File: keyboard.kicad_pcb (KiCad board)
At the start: 2 copper layers, 100 parts, among them J1 AudioJack4, J2 AudioJack4, SW1 , SW11 , SW12 , SW13 , SW14 , SW15 , SW16 , SW17 , SW18 RotaryEncoder_Switch, SW19 , SW2 , SW20 , SW21 , SW22 , SW23 , SW24 SW_PUSH, SW25 SW_PUSH, SW3 , SW4 , SW5 , SW6 , SW7 , SW8 , SW9 , U1 ProMicro

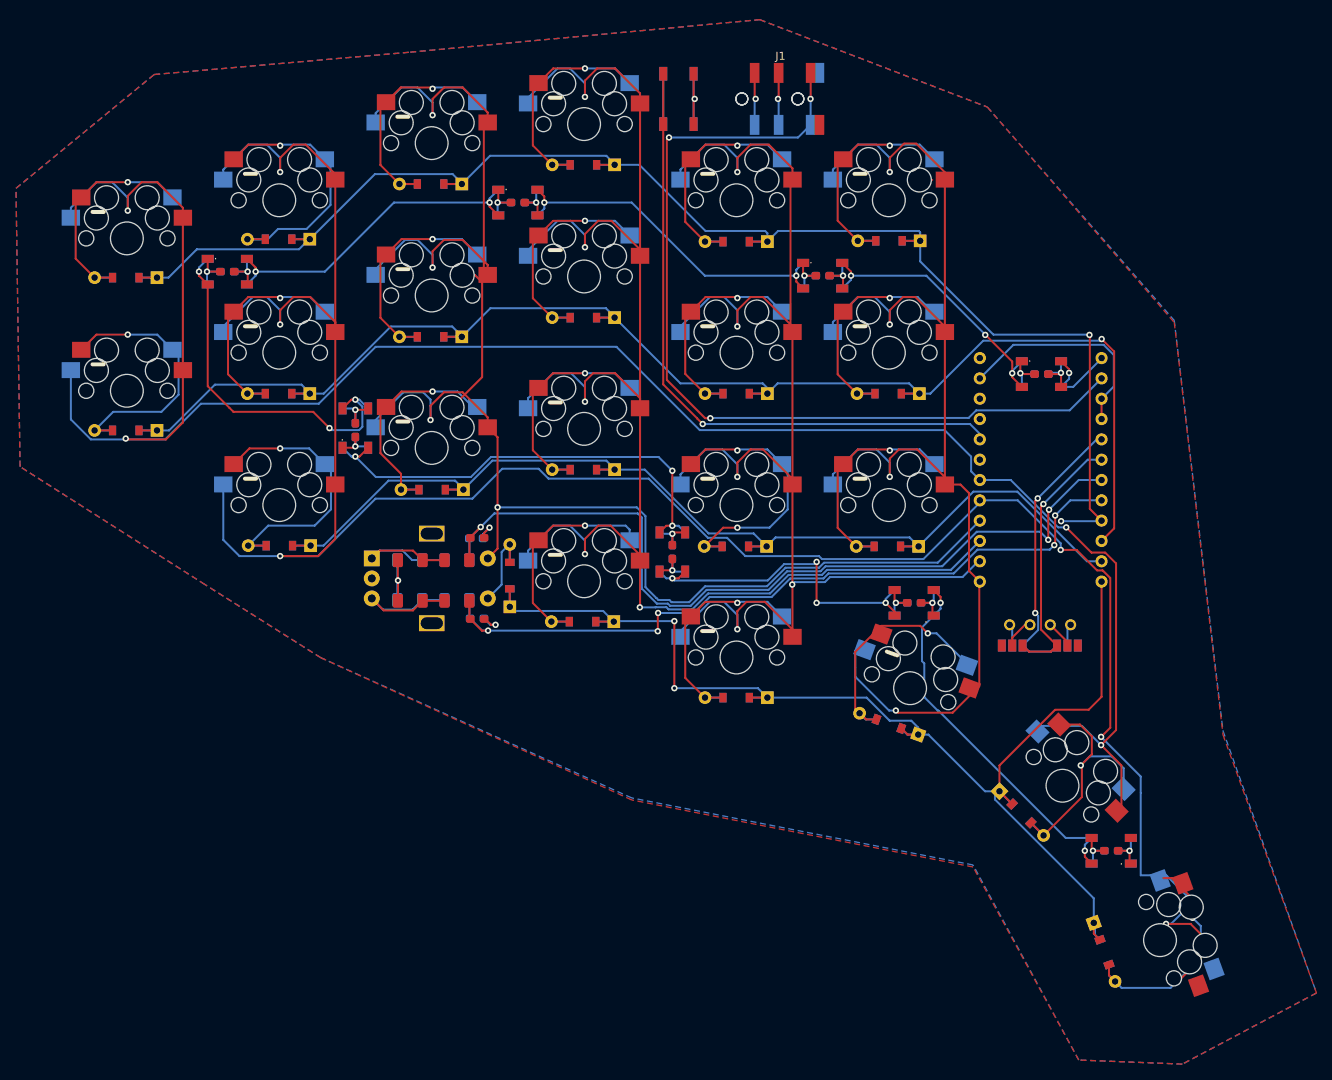
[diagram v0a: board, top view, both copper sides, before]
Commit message: wireless
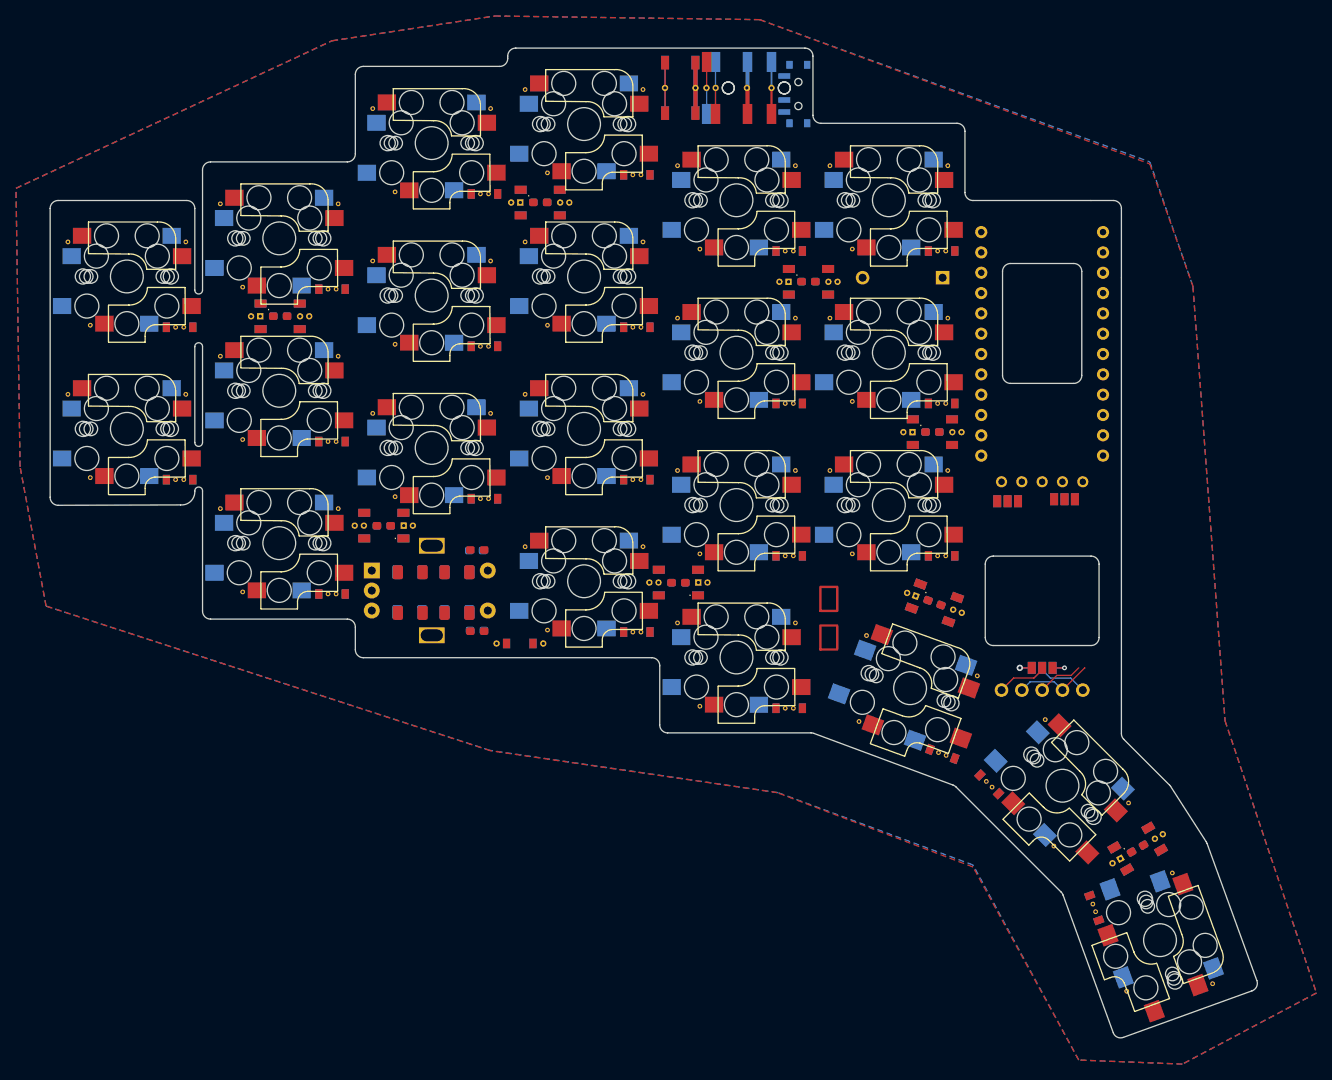
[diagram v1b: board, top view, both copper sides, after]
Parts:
- removed C10, C11, C12, C13, C14, C15, C16, C17, C18, C3, C4, C5, C6, C7, C8, C9: 0.1u, keyswitches:Cap_0603_Clean
- removed D10, D11, D12, D13, D14, D15, D16, D17, D18, D19, D20, D21, D22, D23: , keyswitches:REVERSIBLED_SOD-123
- removed D24, D25, D26, D27, D28, D29, D30, D31, D33, D34, D35, D36, D37, D38, D39, D40: , keyswitches:ledClean
- added J3: Conn_01x05, hb44:Pimoroni Haptic Buzz DRV2605L Driver, B.Cu at (152.1, 99.1)
- added JP5: SolderJumper_3_Open, keyswitches:jumperClean, B.Cu at (152.1, 106.7)
- added JP6: SolderJumper_3_Open, keyswitches:jumperClean, F.Cu at (152.1, 106.7)
- D1: footprint keyswitches:REVERSIBLED_SOD-123 -> hb44:SMD_SOD123
- D2, D3, D4, D5, D6, D7, D8, D9: value (none) -> WS2812B+Cap; footprint keyswitches:REVERSIBLED_SOD-123 -> hb44:SMD_WS2812B+Cap0603; moved to B.Cu
- J1: footprint keyswitches:jackClean -> hb44:SMD_3.5mm_TRRS; moved to B.Cu
- J2: value AudioJack4 -> Conn_01x02; footprint keyswitches:jackClean -> hb44:TH_BatteryConn; moved to F.Cu
- LCD1: renamed from OL1; footprint kbd:OLED_v2 -> hb44:nice!view
- SW1, SW11, SW12, SW13, SW14, SW15, SW16, SW17, SW19, SW2, SW20, SW21, SW3, SW4, SW5, SW6, SW7, SW8, SW9: value (none) -> Switch+Diode; footprint kbd:CherryMX_MidHeight_Hotswap -> hb44:SMD_CherryMX_MidHeight_Choc_HotSwap+SOD123; moved to F.Cu
- SW10: renamed from SWe; value (none) -> Switch+Diode; footprint kbd:CherryMX_MidHeight_Hotswap -> hb44:SMD_CherryMX_MidHeight_Choc_HotSwap+SOD123; moved to F.Cu
- SW22, SW23: value (none) -> Switch+Diode; footprint kbd:CherryMX_MidHeight_Hotswap -> hb44:SMD_CherryMX_MidHeight_Choc_HotSwap+SOD123; moved to B.Cu
- SW24: footprint keyswitches:resetClean -> hb44:SMD_SW_PUSH
- SW25: value SW_PUSH -> SW_DPDT_x2; footprint keyswitches:resetClean -> Button_Switch_SMD:SW_SPDT_PCM12
- U1: value ProMicro -> ProMicro_r; footprint keyswitches:ProMicro_v3Clean -> hb44:nice!nano; moved to B.Cu
- moved D9 108.8 mm to (164.1, 129.3), turned to 30 degrees
- moved D8 85.8 mm to (138.7, 98.6), turned to -20 degrees
- moved D2 85.0 mm to (138.4, 77.2)
- moved D6 72.4 mm to (69.8, 88.9), turned to 180 degrees
- moved D7 71.4 mm to (106.7, 96.0), turned to 180 degrees
- moved D1 66.5 mm to (86.7, 103.2), turned to 180 degrees
- moved D5 57.8 mm to (56.9, 62.7)
- moved D3 48.6 mm to (122.9, 58.4)
- moved J2 30.2 mm to (139.7, 57.9), turned to 180 degrees
- moved JP3 18.3 mm to (154.9, 85.6)
- moved JP4 18.3 mm to (154.9, 85.6)
- moved JP1 18.0 mm to (147.8, 85.9)
- moved JP2 18.0 mm to (147.8, 85.9)
- moved LCD1 17.9 mm to (152.1, 83.4)
- moved U1 15.7 mm to (152.1, 66.7), turned to 180 degrees
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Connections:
- net OLED_1 renamed LCD_1
- net OLED_2 renamed LCD_2
- D1 pad 1: row0 -> row3
- D1 pad 2: Net-(D1-Pad2) -> rotS1
- D2 pad 1: row0 -> VCC
- D3 pad 1: row0 -> VCC
- D4 pad 1: row0 -> VCC
- D5 pad 1: row0 -> VCC
- D6 pad 1: row0 -> VCC
- D7 pad 1: row1 -> VCC
- D8 pad 1: row1 -> VCC
- D9 pad 1: row1 -> VCC
- D9 pad 2: Net-(D9-Pad2) -> unconnected-(D9-Pad2)
- J1 pad T: Data -> CS
- JP1 pad 1: SDA -> MOSI
- JP1 pad 3: GND -> CS
- JP2 pad 1: SCL -> SCK
- JP2 pad 3: VCC -> GND
- JP3 pad 1: VCC -> GND
- JP3 pad 2: OLED_3 -> LCD_4
- JP3 pad 3: SCL -> SCK
- JP4 pad 1: GND -> CS
- JP4 pad 2: OLED_4 -> LCD_5
- JP4 pad 3: SDA -> MOSI
- LCD1 pad 3: OLED_3 -> VCC
- LCD1 pad 4: OLED_4 -> LCD_4
- SW1 pad 2: Net-(D1-Pad2) -> Net-(SW1-Pad2)
- SW2 pad 2: Net-(D2-Pad2) -> Net-(SW2-Pad2)
- SW25 pad 1: Reset -> unconnected-(SW25-Pad1)
- SW25 pad 2: GND -> RAW
- SW3 pad 2: Net-(D3-Pad2) -> Net-(SW3-Pad2)
- SW4 pad 2: Net-(D4-Pad2) -> Net-(SW4-Pad2)
- SW5 pad 2: Net-(D5-Pad2) -> Net-(SW5-Pad2)
- SW6 pad 2: Net-(D6-Pad2) -> Net-(SW6-Pad2)
- SW7 pad 2: Net-(D7-Pad2) -> Net-(SW7-Pad2)
- SW8 pad 2: Net-(D8-Pad2) -> Net-(SW8-Pad2)
- SW9 pad 2: Net-(D9-Pad2) -> Net-(SW9-Pad2)
- U1 pad 19: unconnected-(U1-Pad19) -> rotB
- U1 pad 2: Data -> CS
- U1 pad 20: unconnected-(U1-Pad20) -> rotA
- U1 pad 24: unconnected-(U1-Pad24) -> RAW
- U1 pad 5: SDA -> MOSI
- U1 pad 6: SCL -> SCK
- U1 pad 7: rotA -> SDA
- U1 pad 8: rotB -> SCL
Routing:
- net col1: track 299.5 -> 0.00 mm, vias 6 -> 0
- net col0: track 255.1 -> 0.00 mm, vias 4 -> 0
- net col3: track 205.0 -> 0.00 mm, vias 5 -> 0
- net col2: track 203.6 -> 0.00 mm, vias 4 -> 0
- net row0: track 193.2 -> 0.00 mm, vias 2 -> 0
- net row1: track 188.9 -> 0.00 mm, vias 1 -> 0
- net col4: track 177.4 -> 0.00 mm, vias 5 -> 0
- net col5: track 162.0 -> 0.00 mm, vias 4 -> 0
- net row3: track 159.9 -> 0.00 mm, vias 2 -> 0
- net row2: track 138.8 -> 0.00 mm
- net Data: track 113.7 -> 0.00 mm, vias 3 -> 0
- net rotA: track 107.3 -> 0.00 mm, vias 3 -> 0
- net rotB: track 97.3 -> 0.00 mm, vias 5 -> 0
- net GND: track 103.4 -> 22.2 mm, vias 12 -> 1
- net RESET: track 80.9 -> 12.6 mm, vias 1 -> 0
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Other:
- board outline added: 150.9 x 123.7 mm
- board text added: "失 恋"
